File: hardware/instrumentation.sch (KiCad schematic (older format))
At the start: 19 parts, among them U2 TMUX1309, U3 TMUX1309, U4 LMV554

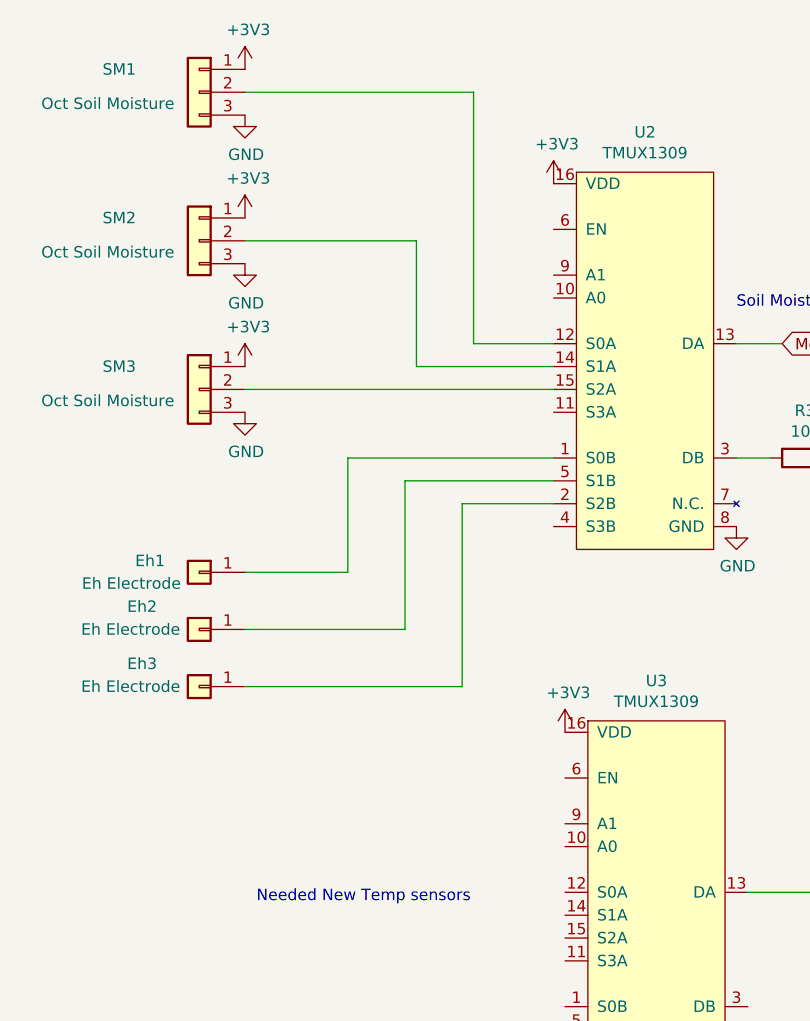
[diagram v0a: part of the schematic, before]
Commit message: Finished MC design
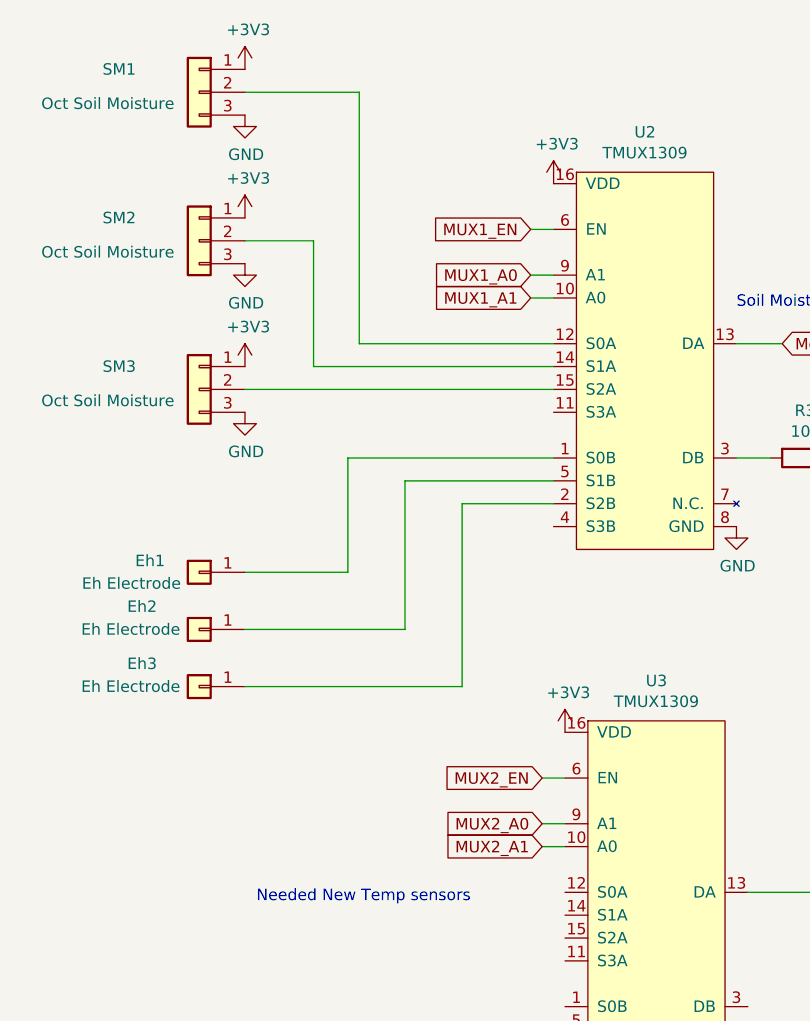
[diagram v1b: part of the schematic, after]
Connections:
- net MUX1_A1: now reaches U2.10 (A0)
- net MUX1_EN: now reaches U2.6 (EN)
- net MUX1_A0: now reaches U2.9 (A1)
- net MUX2_A1: now reaches U3.10 (A0)
- net MUX2_EN: now reaches U3.6 (EN)
- net MUX2_A0: now reaches U3.9 (A1)
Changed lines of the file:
@@
 	2800 2550 4150 2550
 Wire Wire Line
-	3550 1900 3550 2450
-Wire Wire Line
-	3800 1250 3800 2350
+	3100 1900 3100 2450
+Wire Wire Line
+	3300 1250 3300 2350
 Wire Wire Line
 	2800 3350 3250 3350
@@
 	3750 3050 4150 3050
 Wire Wire Line
-	3800 2350 4150 2350
-Wire Wire Line
-	2800 1250 3800 1250
-Wire Wire Line
-	3550 2450 4150 2450
-Wire Wire Line
-	2800 1900 3550 1900
+	3300 2350 4150 2350
+Wire Wire Line
+	2800 1250 3300 1250
+Wire Wire Line
+	3100 2450 4150 2450
+Wire Wire Line
+	2800 1900 3100 1900
 Wire Wire Line
 	5100 2850 4950 2850
@@
 Text Notes 2850 4800 0    50   ~ 0
 Needed New Temp sensors\n
+Text GLabel 4050 1850 0    50   Input ~ 0
+MUX1_EN
+Text GLabel 4050 2050 0    50   Input ~ 0
+MUX1_A0
+Text GLabel 4050 2150 0    50   Input ~ 0
+MUX1_A1
+Wire Wire Line
+	4150 1850 4050 1850
+Wire Wire Line
+	4150 2050 4050 2050
+Wire Wire Line
+	4150 2150 4050 2150
+Text GLabel 4100 4250 0    50   Input ~ 0
+MUX2_EN
+Wire Wire Line
+	4100 4250 4200 4250
+Text GLabel 4100 4450 0    50   Input ~ 0
+MUX2_A0
+Text GLabel 4100 4550 0    50   Input ~ 0
+MUX2_A1
+Wire Wire Line
+	4200 4450 4100 4450
+Wire Wire Line
+	4200 4550 4100 4550
 $EndSCHEMATC

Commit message: Not sure what changes I made sry
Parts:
- U4: Digikey LMP7721MA/NOPB-ND‎ -> (none)
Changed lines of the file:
@@
 F 2 "" H 7500 1600 50  0001 C CNN
 F 3 "https://www.ti.com/lit/ds/symlink/lmv551.pdf?HQS=dis-dk-null-digikeymode-dsf-pf-null-wwe&ts=1626469395066&ref_url=https%253A%252F%252Fwww.ti.com%252Fgeneral%252Fdocs%252Fsuppproductinfo.tsp%253FdistId%253D10%2526gotoUrl%253Dhttps%253A%252F%252Fwww.ti.com%252Flit%252Fgpn%252Flmv551" H 7500 1600 50  0001 C CNN
-F 4 "LMP7721MA/NOPB-ND‎" H 7500 2500 50  0001 C CNN "Digikey"
+F 4 "" H 7500 2500 50  0001 C CNN "Digikey"
 	1    7500 2500
 	1    0    0    -1
